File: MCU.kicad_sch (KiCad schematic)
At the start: 21 parts, among them U7 STM32F405RGTx, U8 8Mhz,50ppm

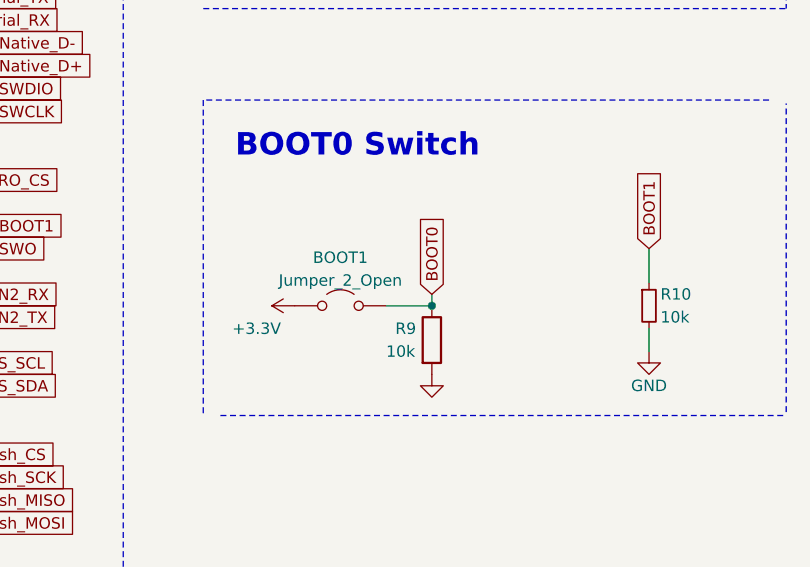
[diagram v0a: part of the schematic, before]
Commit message: update
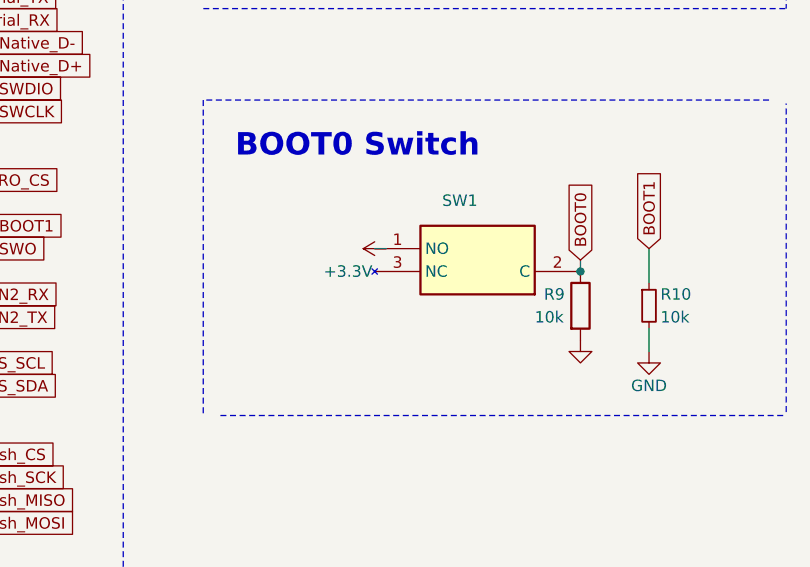
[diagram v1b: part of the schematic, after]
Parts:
- removed BOOT1: Jumper_2_Open, Connector_PinHeader_2.54mm:PinHeader_1x02_P2.54mm_Vertical, symbol Jumper:Jumper_2_Open
- added SW1: SSSS213000, mylib:SSSS213000, symbol SSSS213000:SSSS213000
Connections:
- net +3.3V: now also SW1.1 (NO)
- net BOOT0: now also SW1.2 (C)
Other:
- moved on the sheet: R9
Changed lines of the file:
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@@
 	)
 	(junction
-		(at 154.94 148.59)
-		(diameter 0)
-		(color 0 0 0 0)
-	)
-	(junction
 		(at 69.85 53.34)
 		(diameter 0)
@@
 	)
 	(junction
+		(at 171.45 144.78)
+		(diameter 0)
+		(color 0 0 0 0)
+	)
+	(junction
 		(at 148.59 45.72)
 		(diameter 0)
@@
 	(wire
 		(pts
+			(xy 148.59 142.24) (xy 149.86 142.24)
+		)
+		(stroke
+			(width 0)
+			(type default)
+		)
+	)
+	(wire
+		(pts
 			(xy 250.19 134.62) (xy 250.19 138.43)
 		)
@@
 	(wire
 		(pts
-			(xy 154.94 147.32) (xy 154.94 148.59)
+			(xy 171.45 143.51) (xy 171.45 144.78)
 		)
 		(stroke
@@
 	(wire
 		(pts
-			(xy 149.86 148.59) (xy 154.94 148.59)
-		)
-		(stroke
-			(width 0)
-			(type default)
-		)
-	)
-	(wire
-		(pts
 			(xy 90.17 81.28) (xy 90.17 83.82)
 		)
@@
 	(global_label "BOOT0"
 		(shape input)
-		(at 154.94 147.32 90)
+		(at 171.45 143.51 90)
 		(effects
 			(font
@@
 		)
 		(property "Intersheetrefs" "${INTERSHEET_REFS}"
-			(at 154.94 147.32 90)
+			(at 171.45 143.51 90)
 			(effects
 				(font
@@
 		(on_board yes)
 		(dnp no)
-		(property "Reference" "#PWR051"
+		(property "Reference" "#PWR050"
 			(at 148.59 49.53 0)
 			(effects
@@
 			(project "MX_IMU"
 				(path "/8ed38441-7d4e-4e89-870f-07e11c6dce38/39c93069-edc2-4035-8fc7-27a45736847d"
-					(reference "#PWR051")
+					(reference "#PWR050")
 					(unit 1)
 				)
@@
 	)
 	(symbol
+		(lib_id "SSSS213000:SSSS213000")
+		(at 171.45 144.78 180)
+		(unit 1)
+		(exclude_from_sim no)
+		(in_bom yes)
+		(on_board yes)
+		(dnp no)
+		(property "Reference" "SW1"
+			(at 160.02 136.906 0)
+			(effects
+				(font
+					(size 1.27 1.27)
+				)
+				(justify left)
+			)
+		)
+		(property "Value" "SSSS213000"
+			(at 160.0201 157.48 90)
+			(effects
+				(font
+					(size 1.27 1.27)
+				)
+				(justify left)
+				(hide yes)
+			)
+		)
+		(property "Footprint" "mylib:SSSS213000"
+			(at 152.4 49.86 0)
+			(effects
+				(font
+					(size 1.27 1.27)
+				)
+				(justify left top)
+				(hide yes)
+			)
+		)
+		(property "Datasheet" "https://www.alps.com/prod/info/E/HTML/Switch/Slide/SSSS2/SSSS213000.html"
+			(at 152.4 -50.14 0)
+			(effects
+				(font
+					(size 1.27 1.27)
+				)
+				(justify left top)
+				(hide yes)
+			)
+		)
+		(property "Description" "Slide Switches 1-pole 2-positions"
+			(at 171.45 144.78 0)
+			(effects
+				(font
+					(size 1.27 1.27)
+				)
+				(hide yes)
+			)
+		)
+		(property "Height" "5"
+			(at 152.4 -250.14 0)
+			(effects
+				(font
+					(size 1.27 1.27)
+				)
+				(justify left top)
+				(hide yes)
+			)
+		)
+		(property "Avnet Part Number" ""
+			(at 152.4 -350.14 0)
+			(effects
+				(font
+					(size 1.27 1.27)
+				)
+				(justify left top)
+				(hide yes)
+			)
+		)
+		(property "Avnet Price/Stock" ""
+			(at 152.4 -450.14 0)
+			(effects
+				(font
+					(size 1.27 1.27)
+				)
+				(justify left top)
+				(hide yes)
+			)
+		)
+		(property "Manufacturer_Name" "ALPS Electric"
+			(at 152.4 -550.14 0)
+			(effects
+				(font
+					(size 1.27 1.27)
+				)
+				(justify left top)
+				(hide yes)
+			)
+		)
+		(property "Manufacturer_Part_Number" "SSSS213000"
+			(at 152.4 -650.14 0)
+			(effects
+				(font
+					(size 1.27 1.27)
+				)
+				(justify left top)
+				(hide yes)
+			)
+		)
+		(pin "3"
+		)
+		(pin "1"
+		)
+		(pin "2"
+		)
+		(instances
+			(project "MX_IMU"
+				(path "/8ed38441-7d4e-4e89-870f-07e11c6dce38/39c93069-edc2-4035-8fc7-27a45736847d"
+					(reference "SW1")
+					(unit 1)
+				)
+			)
+		)
+	)
+	(symbol
 		(lib_id "Device:C_Small")
 		(at 243.84 143.51 180)
@@
 		(on_board yes)
 		(dnp no)
-		(property "Reference" "#PWR054"
+		(property "Reference" "#PWR053"
 			(at 168.91 85.09 0)
 			(effects
@@
 			(project "MX_IMU"
 				(path "/8ed38441-7d4e-4e89-870f-07e11c6dce38/39c93069-edc2-4035-8fc7-27a45736847d"
-					(reference "#PWR054")
+					(reference "#PWR053")
 					(unit 1)
 				)
@@
 	)
 	(symbol
-		(lib_id "Jumper:Jumper_2_Open")
-		(at 144.78 148.59 0)
-		(unit 1)
-		(exclude_from_sim no)
-		(in_bom yes)
-		(on_board yes)
-		(dnp no)
-		(property "Reference" "BOOT1"
-			(at 144.78 143.2392 0)
-			(effects
-				(font
-					(size 1.27 1.27)
-				)
-			)
-		)
-		(property "Value" "Jumper_2_Open"
-			(at 144.78 145.7761 0)
-			(effects
-				(font
-					(size 1.27 1.27)
-				)
-			)
-		)
-		(property "Footprint" "Connector_PinHeader_2.54mm:PinHeader_1x02_P2.54mm_Vertical"
-			(at 144.78 148.59 0)
-			(effects
-				(font
-					(size 1.27 1.27)
-				)
-				(hide yes)
-			)
-		)
-		(property "Datasheet" "~"
-			(at 144.78 148.59 0)
-			(effects
-				(font
-					(size 1.27 1.27)
-				)
-				(hide yes)
-			)
-		)
-		(property "Description" ""
-			(at 144.78 148.59 0)
-			(effects
-				(font
-					(size 1.27 1.27)
-				)
-			)
-		)
-		(pin "1"
-		)
-		(pin "2"
-		)
-		(instances
-			(project "MX_IMU"
-				(path "/8ed38441-7d4e-4e89-870f-07e11c6dce38/39c93069-edc2-4035-8fc7-27a45736847d"
-					(reference "BOOT1")
-					(unit 1)
-				)
-			)
-		)
-	)
-	(symbol
 		(lib_id "power:PWR_FLAG")
 		(at 140.97 45.72 0)
@@
 	(symbol
 		(lib_id "power:+3.3V")
-		(at 139.7 148.59 90)
+		(at 149.86 142.24 90)
 		(unit 1)
 		(exclude_from_sim no)
@@
 		(on_board yes)
 		(dnp no)
-		(property "Reference" "#PWR050"
-			(at 143.51 148.59 0)
+		(property "Reference" "#PWR051"
+			(at 153.67 142.24 0)
 			(effects
 				(font
@@
 		)
 		(property "Value" "+3.3V"
-			(at 138.176 151.13 90)
+			(at 148.336 144.78 90)
 			(effects
 				(font
@@
 		)
 		(property "Footprint" ""
-			(at 139.7 148.59 0)
+			(at 149.86 142.24 0)
 			(effects
 				(font
@@
 		)
 		(property "Datasheet" ""
-			(at 139.7 148.59 0)
+			(at 149.86 142.24 0)
 			(effects
 				(font
@@
 		)
 		(property "Description" "Power symbol creates a global label with name \"+3.3V\""
-			(at 139.7 148.59 0)
+			(at 149.86 142.24 0)
 			(effects
 				(font
@@
 			(project "MX_IMU"
 				(path "/8ed38441-7d4e-4e89-870f-07e11c6dce38/39c93069-edc2-4035-8fc7-27a45736847d"
-					(reference "#PWR050")
+					(reference "#PWR051")
 					(unit 1)
 				)
@@
 		(dnp no)
 		(fields_autoplaced yes)
-		(property "Reference" "#PWR055"
+		(property "Reference" "#PWR054"
 			(at 165.1 111.76 0)
 			(effects
@@
 			(project "MX_IMU"
 				(path "/8ed38441-7d4e-4e89-870f-07e11c6dce38/39c93069-edc2-4035-8fc7-27a45736847d"
-					(reference "#PWR055")
+					(reference "#PWR054")
 					(unit 1)
 				)
@@
 	(symbol
 		(lib_id "power:GND")
-		(at 154.94 156.21 0)
+		(at 171.45 152.4 0)
 		(unit 1)
 		(exclude_from_sim no)
@@
 		(dnp no)
 		(fields_autoplaced yes)
-		(property "Reference" "#PWR053"
-			(at 154.94 162.56 0)
+		(property "Reference" "#PWR055"
+			(at 171.45 158.75 0)
 			(effects
 				(font
@@
 		)
 		(property "Value" "GND"
-			(at 154.94 161.29 0)
+			(at 171.45 157.48 0)
 			(effects
 				(font
@@
 		)
 		(property "Footprint" ""
-			(at 154.94 156.21 0)
+			(at 171.45 152.4 0)
 			(effects
 				(font
@@
 		)
 		(property "Datasheet" ""
-			(at 154.94 156.21 0)
+			(at 171.45 152.4 0)
 			(effects
 				(font
@@
 		)
 		(property "Description" "Power symbol creates a global label with name \"GND\" , ground"
-			(at 154.94 156.21 0)
+			(at 171.45 152.4 0)
 			(effects
 				(font
@@
 			(project "MX_IMU"
 				(path "/8ed38441-7d4e-4e89-870f-07e11c6dce38/39c93069-edc2-4035-8fc7-27a45736847d"
-					(reference "#PWR053")
+					(reference "#PWR055")
 					(unit 1)
 				)
@@
 	(symbol
 		(lib_id "Device:R")
-		(at 154.94 152.4 0)
+		(at 171.45 148.59 0)
 		(unit 1)
 		(exclude_from_sim no)
@@
 		(dnp no)
 		(property "Reference" "R9"
-			(at 150.876 151.13 0)
+			(at 167.386 147.32 0)
 			(effects
 				(font
@@
 		)
 		(property "Value" "10k"
-			(at 149.86 153.67 0)
+			(at 166.37 149.86 0)
 			(effects
 				(font
@@
 		)
 		(property "Footprint" "Resistor_SMD:R_0603_1608Metric"
-			(at 153.162 152.4 90)
+			(at 169.672 148.59 90)
 			(effects
 				(font
@@
 		)
 		(property "Datasheet" "~"
-			(at 154.94 152.4 0)
+			(at 171.45 148.59 0)
 			(effects
 				(font
@@
 		)
 		(property "Description" "Resistor"
-			(at 154.94 152.4 0)
+			(at 171.45 148.59 0)
 			(effects
 				(font

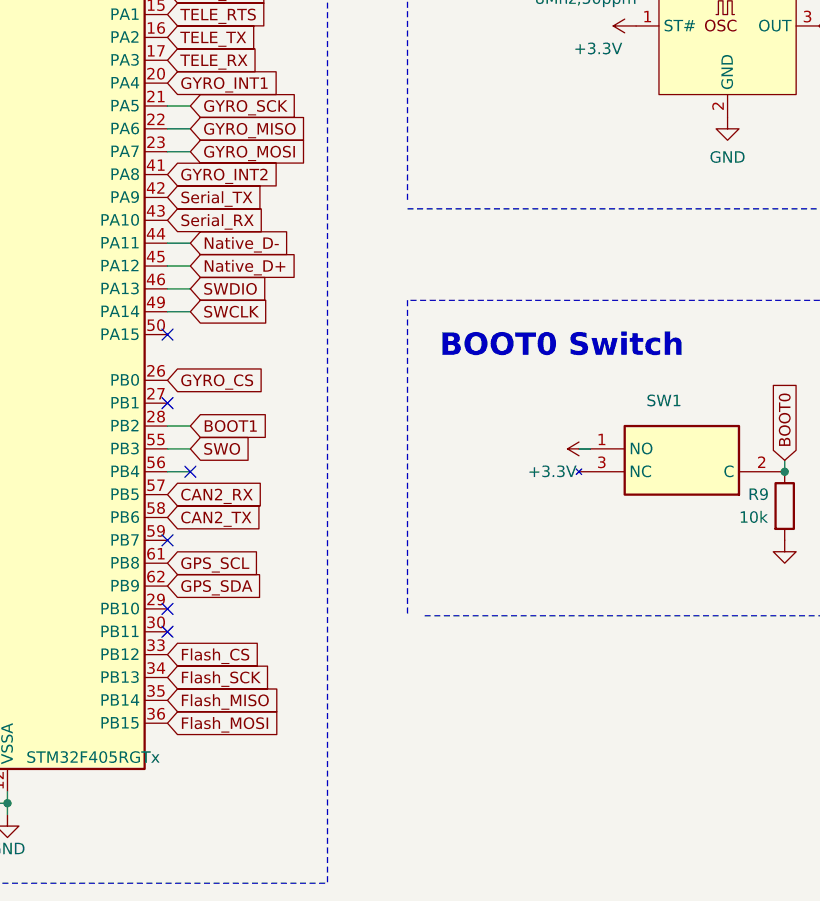
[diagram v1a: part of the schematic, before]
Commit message: update
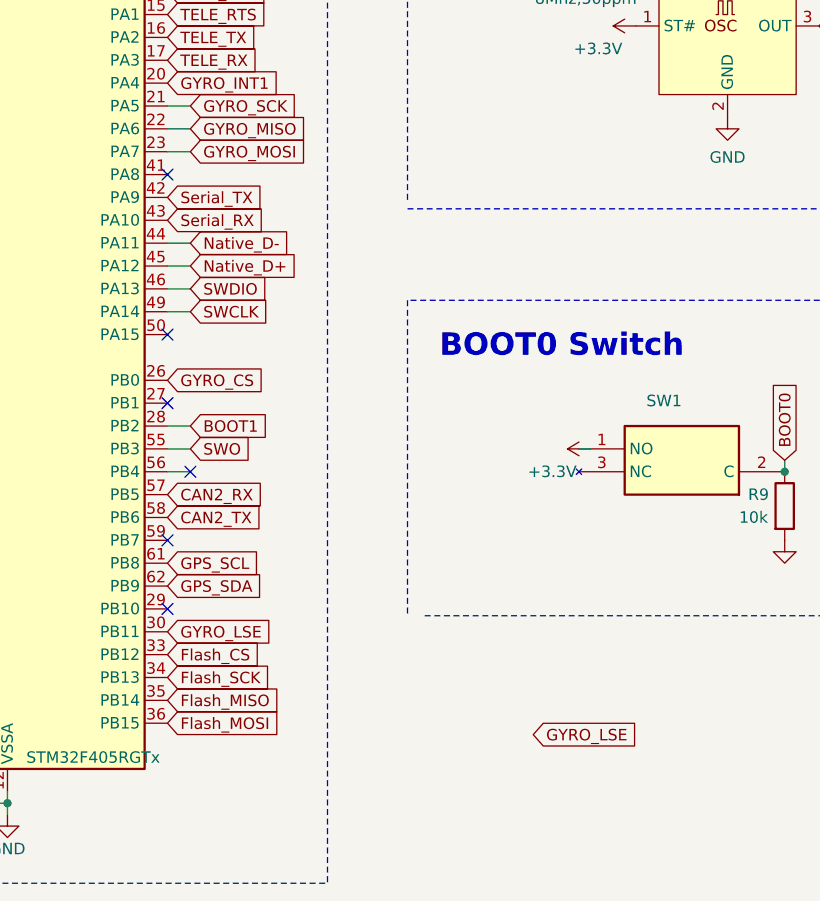
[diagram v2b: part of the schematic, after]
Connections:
- net GYRO_LSE: now reaches U7.30 (PB11)
- net GYRO_INT2: no longer names the net of U7.41 (PA8)
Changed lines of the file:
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@@
+	)
+	(no_connect
+		(at 102.87 111.76)
 	)
 	(no_connect
 		(at 62.23 116.84)
-	)
-	(no_connect
-		(at 102.87 162.56)
 	)
 	(no_connect
@@
 		)
 	)
+	(global_label "GYRO_LSE"
+		(shape input)
+		(at 102.87 162.56 0)
+		(effects
+			(font
+				(size 1.27 1.27)
+			)
+			(justify left)
+		)
+		(property "Intersheetrefs" "${INTERSHEET_REFS}"
+			(at 102.87 162.56 0)
+			(effects
+				(font
+					(size 1.27 1.27)
+				)
+				(hide yes)
+			)
+		)
+	)
 	(global_label "GPS_RX"
 		(shape input)
@@
 		(property "Intersheetrefs" "${INTERSHEET_REFS}"
 			(at 62.23 142.24 0)
+			(effects
+				(font
+					(size 1.27 1.27)
+				)
+				(hide yes)
+			)
+		)
+	)
+	(global_label "GYRO_LSE"
+		(shape input)
+		(at 143.51 173.99 0)
+		(effects
+			(font
+				(size 1.27 1.27)
+			)
+			(justify left)
+		)
+		(property "Intersheetrefs" "${INTERSHEET_REFS}"
+			(at 143.51 173.99 0)
 			(effects
 				(font
@@
 				(hide yes)
 			)
-		)
-	)
-	(global_label "GYRO_INT2"
-		(shape input)
-		(at 102.87 111.76 0)
-		(effects
-			(font
-				(size 1.27 1.27)
-			)
-			(justify left)
-		)
-		(property "Intersheetrefs" "${INTERSHEET_REFS}"
-			(at 102.87 111.76 0)
-			(effects
-				(font
-					(size 1.27 1.27)
-				)
-				(hide yes)
-			)
